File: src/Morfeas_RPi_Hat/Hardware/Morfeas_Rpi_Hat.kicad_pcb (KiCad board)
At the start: 2 copper layers, 65 x 56 mm, 52 parts, among them J1 Power IN, J2 RPi_header, J3 CAN0_Power+, J4 CAN1_Power+, J5 RS_232, Q1 SUM110P06, Q2 SUM110P06, U1 DS3231, U2 TSR2-2450, U3 TLV70433, U4 SP3232, U5 24AA08, U6 MAX9611, U7 MAX9611

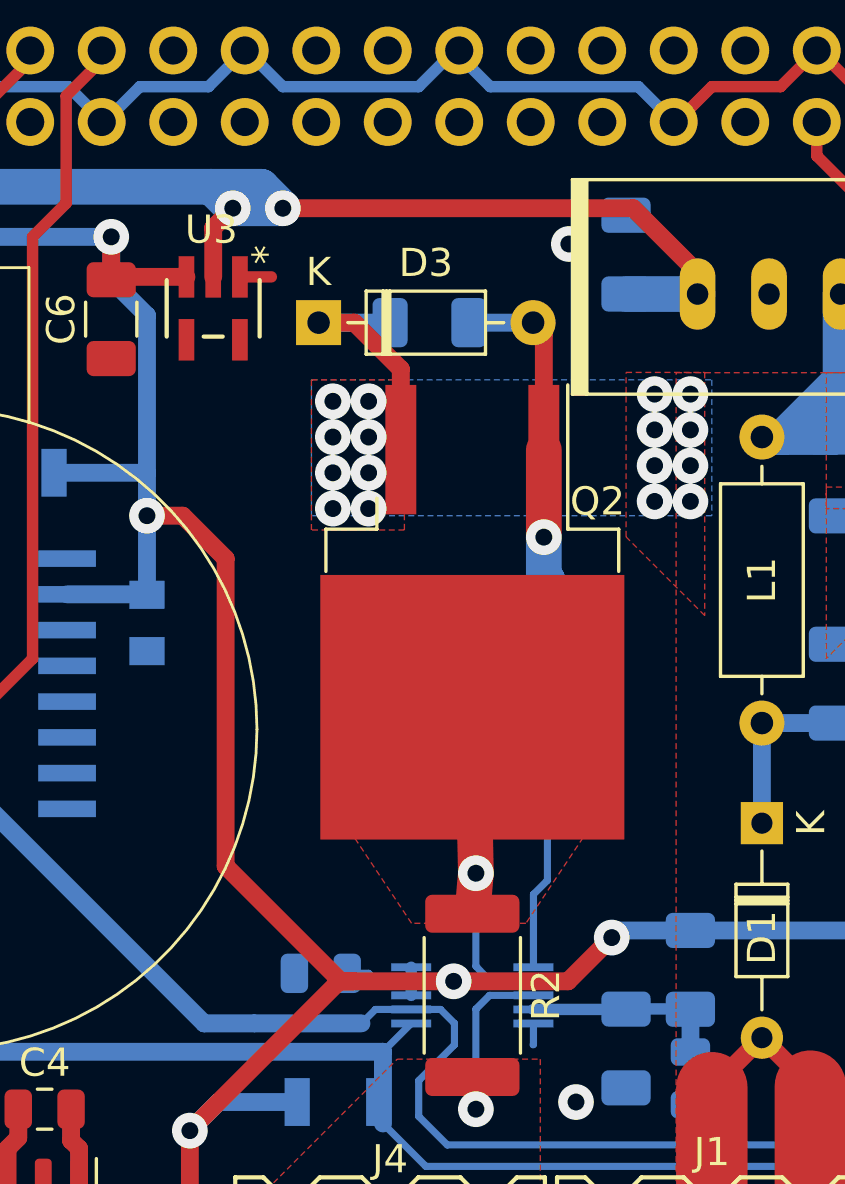
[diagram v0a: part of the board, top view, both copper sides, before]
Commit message: Update Morfeas_RPi_hat
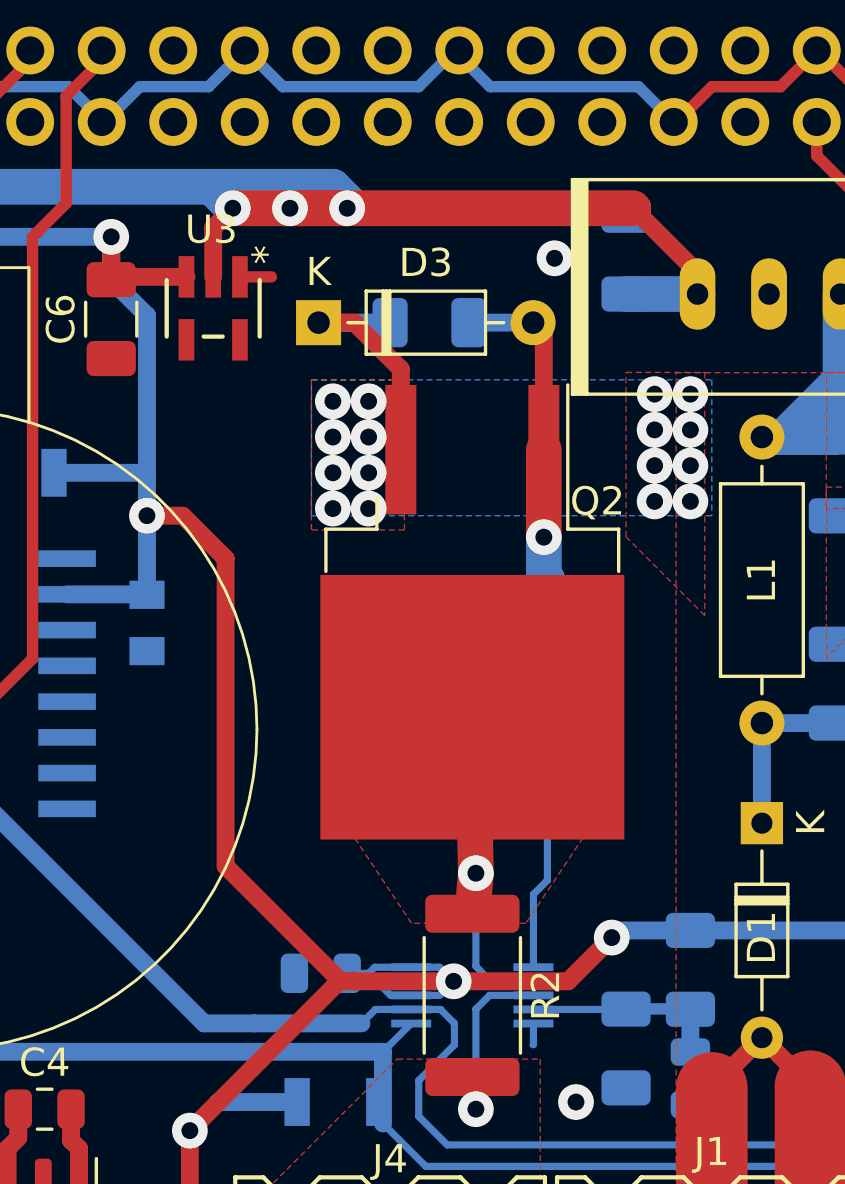
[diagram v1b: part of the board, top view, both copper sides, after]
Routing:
- net +5V: track 52.6 -> 61.7 mm, vias 2 -> 3
- net +3V3: track 132.3 -> 137.8 mm
- net Net-(C12-Pad2): track 7.01 -> 7.51 mm
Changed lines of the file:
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@@
     (thickness 1.6)
     (drawings 21)
-    (tracks 351)
+    (tracks 362)
     (zones 0)
     (modules 52)
@@
   )
   (layers
-    (0 F.Cu signal)
+    (0 F.Cu signal hide)
     (31 B.Cu signal)
     (32 B.Adhes user hide)
     (33 F.Adhes user hide)
-    (34 B.Paste user)
-    (35 F.Paste user)
-    (36 B.SilkS user)
-    (37 F.SilkS user)
+    (34 B.Paste user hide)
+    (35 F.Paste user hide)
+    (36 B.SilkS user hide)
+    (37 F.SilkS user hide)
     (38 B.Mask user)
-    (39 F.Mask user)
+    (39 F.Mask user hide)
     (40 Dwgs.User user)
     (41 Cmts.User user)
@@
   )
   (setup
-    (last_trace_width 1.27)
+    (last_trace_width 0.254)
     (user_trace_width 0.4064)
     (user_trace_width 0.635)
@@
   (segment (start 83.917 107.031) (end 85.09 107.031) (width 0.635) (layer B.Cu) (net 1) (status 10))
   (segment (start 85.078 106.922) (end 85.949 106.075) (width 0.635) (layer B.Cu) (net 1))
-  (via (at 103.124 70.104) (size 1.27) (drill 0.6) (layers F.Cu B.Cu) (net 1))
+  (via (at 102.616 70.612) (size 1.27) (drill 0.6) (layers F.Cu B.Cu) (net 1))
   (segment (start 99.076 63.23) (end 97.79 64.516) (width 0.4064) (layer B.Cu) (net 1) (status 10))
   (segment (start 99.23 63.23) (end 99.076 63.23) (width 0.4064) (layer B.Cu) (net 1) (status 30))
@@
   (segment (start 76.37 63.23) (end 78.91 63.23) (width 1.27) (layer B.Cu) (net 5) (status 30))
   (segment (start 107.696 71.12) (end 107.696 71.882) (width 0.635) (layer F.Cu) (net 5) (status 30))
-  (via (at 92.964 68.834) (size 1.27) (drill 0.6) (layers F.Cu B.Cu) (net 5))
-  (segment (start 92.964 68.834) (end 92.202 68.072) (width 1.27) (layer B.Cu) (net 5))
-  (segment (start 92.202 68.072) (end 90.424 68.072) (width 1.27) (layer B.Cu) (net 5))
-  (segment (start 92.964 68.834) (end 105.41 68.834) (width 0.635) (layer F.Cu) (net 5))
+  (via (at 95.25 68.834) (size 1.27) (drill 0.6) (layers F.Cu B.Cu) (net 5))
+  (segment (start 92.964 68.834) (end 105.41 68.834) (width 1.27) (layer F.Cu) (net 5))
   (segment (start 105.41 68.834) (end 107.696 71.12) (width 0.635) (layer F.Cu) (net 5) (status 20))
-  (segment (start 92.964 68.834) (end 91.186 68.834) (width 1.27) (layer B.Cu) (net 5))
   (segment (start 107.696 71.882) (end 105.156 71.882) (width 1.27) (layer B.Cu) (net 5) (status 30))
+  (segment (start 91.186 68.834) (end 92.964 68.834) (width 1.27) (layer B.Cu) (net 5))
+  (segment (start 94.742 68.072) (end 90.424 68.072) (width 1.27) (layer B.Cu) (net 5))
+  (segment (start 92.964 68.834) (end 93.218 68.834) (width 1.27) (layer B.Cu) (net 5))
+  (segment (start 95.504 68.834) (end 94.742 68.072) (width 1.27) (layer B.Cu) (net 5))
+  (segment (start 93.218 68.834) (end 95.504 68.834) (width 1.27) (layer B.Cu) (net 5))
+  (via (at 93.218 68.834) (size 1.27) (drill 0.6) (layers F.Cu B.Cu) (net 5))
+  (segment (start 91.186 68.834) (end 95.25 68.834) (width 1.27) (layer F.Cu) (net 5))
   (segment (start 83.185 102.235) (end 83.185 103.57) (width 0.635) (layer F.Cu) (net 6) (status 20))
   (segment (start 83.566 100.838) (end 83.566 101.854) (width 0.635) (layer F.Cu) (net 6) (status 10))
@@
   (via (at 86.868 69.85) (size 1.27) (drill 0.6) (layers F.Cu B.Cu) (net 10))
   (segment (start 86.868 71.374) (end 86.868 69.85) (width 0.635) (layer F.Cu) (net 10) (status 10))
-  (segment (start 97.5233 95.794999) (end 97.5233 96.795) (width 0.4064) (layer B.Cu) (net 10) (status 30))
-  (segment (start 97.5233 96.295001) (end 99.030999 96.295001) (width 0.4064) (layer B.Cu) (net 10) (status 10))
-  (via (at 99.030999 96.295001) (size 1.27) (drill 0.6) (layers F.Cu B.Cu) (net 10))
   (segment (start 99.030999 96.295001) (end 103.094999 96.295001) (width 0.635) (layer F.Cu) (net 10))
   (segment (start 103.094999 96.295001) (end 104.648 94.742) (width 0.635) (layer F.Cu) (net 10))
@@
   (via (at 89.662 101.6) (size 1.27) (drill 0.6) (layers F.Cu B.Cu) (net 10))
   (segment (start 90.678 100.584) (end 89.662 101.6) (width 0.635) (layer B.Cu) (net 10))
+  (via (at 99.030999 96.295001) (size 1.27) (drill 0.6) (layers F.Cu B.Cu) (net 10))
+  (segment (start 97.5233 96.295001) (end 99.030999 96.295001) (width 0.254) (layer B.Cu) (net 10))
+  (segment (start 98.530997 95.794999) (end 99.030999 96.295001) (width 0.254) (layer B.Cu) (net 10))
+  (segment (start 97.5233 95.794999) (end 98.530997 95.794999) (width 0.254) (layer B.Cu) (net 10))
+  (segment (start 98.531 96.795) (end 99.030999 96.295001) (width 0.254) (layer B.Cu) (net 10))
+  (segment (start 97.5233 96.795) (end 98.531 96.795) (width 0.254) (layer B.Cu) (net 10))
+  (segment (start 96.795 96.795) (end 96.295001 96.295001) (width 0.254) (layer B.Cu) (net 10))
+  (segment (start 97.5233 96.795) (end 96.795 96.795) (width 0.254) (layer B.Cu) (net 10))
+  (segment (start 96.229001 95.794999) (end 96.012 96.012) (width 0.254) (layer B.Cu) (net 10))
+  (segment (start 97.5233 95.794999) (end 96.229001 95.794999) (width 0.254) (layer B.Cu) (net 10))
   (segment (start 84.455 103.57) (end 84.455 105.029) (width 0.254) (layer F.Cu) (net 11) (status 10))
   (segment (start 84.455 105.029) (end 84.074 105.41) (width 0.254) (layer F.Cu) (net 11))
@@
   (segment (start 128.524 99.054) (end 128.524 98.298) (width 1.27) (layer F.Cu) (net 13) (status 10))
   (segment (start 128.524 98.298) (end 128.524 97.282) (width 1.27) (layer F.Cu) (net 13) (status 20))
-  (segment (start 104.629001 97.294999) (end 104.648 97.276) (width 0.4064) (layer B.Cu) (net 14) (status 30))
-  (segment (start 101.8667 97.294999) (end 104.629001 97.294999) (width 0.4064) (layer B.Cu) (net 14) (status 30))
   (segment (start 107.43 97.276) (end 107.442 97.288) (width 0.4064) (layer B.Cu) (net 14) (status 30))
   (segment (start 104.648 97.276) (end 107.43 97.276) (width 0.4064) (layer B.Cu) (net 14) (status 30))
   (segment (start 107.442 97.288) (end 107.442 98.709) (width 0.635) (layer B.Cu) (net 14) (status 30))
+  (segment (start 105.143001 97.294999) (end 105.156 97.282) (width 0.254) (layer B.Cu) (net 14))
+  (segment (start 101.8667 97.294999) (end 105.143001 97.294999) (width 0.254) (layer B.Cu) (net 14))
   (segment (start 95.504 72.898) (end 94.234 72.898) (width 0.635) (layer F.Cu) (net 15) (status 20))
   (segment (start 97.155 74.549) (end 95.504 72.898) (width 0.635) (layer F.Cu) (net 15))
